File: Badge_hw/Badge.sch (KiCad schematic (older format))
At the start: 133 parts, among them Q1 IRLML9303, Q2 NPN, SW1 SW_PUSH

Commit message: update 9.12 - scheme + case updated
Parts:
- removed ANT1: ANT_PCB_MONO, symbol ANT_PCB_MONO
- removed DD4: STM32L476Rx, LQFP_TQFP:LQFP64, symbol STM32L476Rx
- added D4, D5, D6: LED, symbol LED
- added D7: ANT, symbol ANT
- added DD4: STM32L476Vx, LQFP_TQFP:LQFP100, symbol STM32L476Vx
- added R41: 40kR, symbol R-RESCUE-Badge
- added R42, R43, R44, R45: 1kR, symbol R-RESCUE-Badge
- added R?: Fuse0R, symbol R-RESCUE-Badge
- added SA2, SA3: SW_PUSH, symbol SW_PUSH
- C51, C53: value 18pF -> 18p
- D3: symbol DIODE -> DIODE-RESCUE-Badge
- L1, L2, L3, L4, L5, L6, L7: symbol L -> L-RESCUE-Badge
- R2: value 470R -> 1kR
- R31: value 500R -> 1kR
- R35: value 195 -> 195R
- renumbered SW1 to SA1
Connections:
- net labels added: VGND
- net labels removed: GNDD, GNDPWR, MCU_RST
- wire segments 479 -> 516
- no-connect marks 17 -> 44
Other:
- note added: "Battery"
- note added: "I2C PullUp"
- note added: "LCD"
- note added: "POWOK ?"
- note added: "Power supply"
- note added: "RGB LED"
- note removed: "21"
- note removed: "LED"
- moved on the sheet: C1, C10, C11, C12, C13, C15, C16, C17, C18, C19, C2, C21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

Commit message: 9.2 +pcb
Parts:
- removed D4, D5, D6: LED, symbol LED
- added C67: 10u, Capacitors:CAP_0603, symbol C-RESCUE-Badge
- added D4: LED_RGB, LEDs:LED_5050, symbol LED_RGB-RESCUE-Badge
- added TP1: TESTPOINT, PCB:TESTPOINT_1MM, symbol TESTPOINT
- C1, C10, C11, C12, C13, C14, C15, C16, C17, C18, C19, C2, C20, C21, C22, C23, C24, C25, C26, C27, C28, C29, C3, C30, C31, C32, C33, C34, C35, C36, C37, C38, C39, C4, C40, C41, C42, C43, C44, C45, C46, C47, C48, C49, C50, C51, C52, C53, C54, C55, C56, C57, C58, C59, C6, C60, C61, C62, C63, C65, C66, C7, C8, C9: footprint (none) -> Capacitors:CAP_0603
- C5: value 22u -> 10u; footprint (none) -> Capacitors:CAP_0603
- C64: value 3.9pF -> 3.9pF*; footprint (none) -> Capacitors:CAP_0603
- D1, D2: footprint (none) -> LEDs:LED_0603; symbol LED -> LED-RESCUE-Badge
- D3: footprint (none) -> Diodes:SOD80C
- DA1: footprint (none) -> SO_DIL_TSSOP:SO8_208MIL
- DD1: footprint QFN_DFN:QFN16_4x4_H -> LGA:16_4X4_P065
- DD2: footprint (none) -> Connectors:ER-CON50HT-1
- DD3: footprint (none) -> QFN_DFN:QFN48
- L7: value 12nH -> 12nH*
- LIPO_BAT1: footprint (none) -> Connectors:PLS-2
- Q1: footprint (none) -> SOT:SOT23-3
- Q2: value NPN -> BC848; footprint (none) -> SOT:SOT23-3
- R1, R10, R11, R12, R13, R14, R15, R16, R17, R18, R19, R20, R21, R22, R23, R24, R25, R26, R27, R28, R29, R3, R30, R32, R33, R34, R36, R37, R38, R39, R4, R40, R5, R6, R7, R8, R9: footprint (none) -> Resistors:RES_0603
- R2, R31, R42, R43, R44, R45: value 1kR -> 1k; footprint (none) -> Resistors:RES_0603
- R35: value 195R -> 56k; footprint (none) -> Resistors:RES_0603
- R41: value 40kR -> 51k; footprint (none) -> Resistors:RES_0603
- R46: renamed from R?; footprint (none) -> Resistors:RES_0603_FUSE
- SA1, SA2, SA3: footprint (none) -> BtnsSwitches:BTN_6x6_4x4
- XL1: footprint (none) -> Connectors:PLS-6
- XL2: footprint (none) -> Connectors:USBmicro_MOLEX_WM17142
- XL3: footprint (none) -> Connectors:MICROSD_CAP_FIX05A
- XTAL1: footprint (none) -> Quartz:0503x4-4
- XTAL2: footprint CRYSTAL -> Quartz:0503x4-4
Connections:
- net labels added: +3V3
- wire segments 516 -> 520
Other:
- note removed: "Debug LED"
- note removed: "RGB LED"
- moved on the sheet: BLN1, C1, C10, C11, C12, C13, C15, C17, C18, C19, C2, C21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

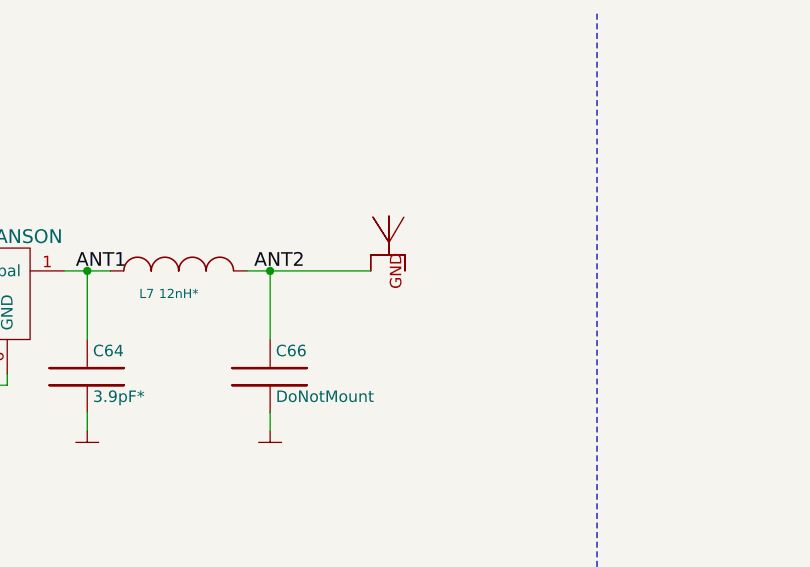
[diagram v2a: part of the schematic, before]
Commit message: +antenna
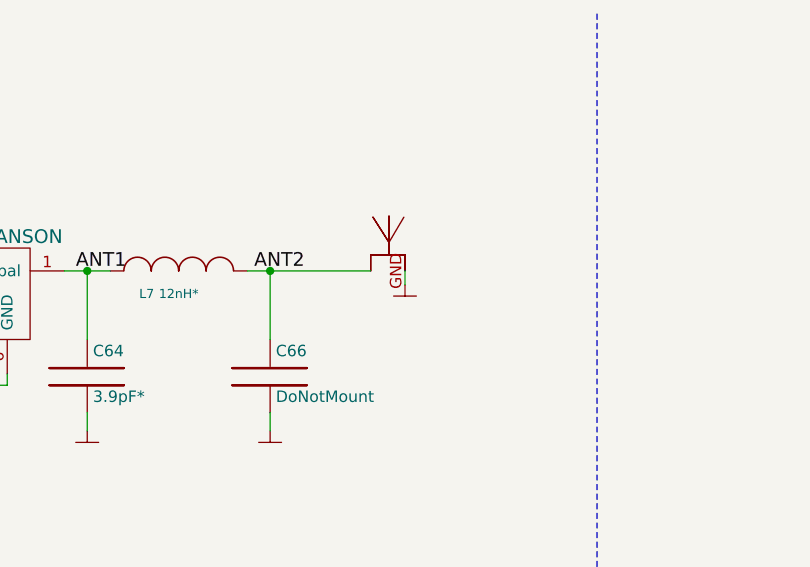
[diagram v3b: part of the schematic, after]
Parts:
- D7: footprint (none) -> ANT_868_INV_F:ANTENNA_868_INV_F
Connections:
- wire segments 520 -> 521
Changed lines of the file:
@@
 LIBS:contrib
 LIBS:valves
-LIBS:ns_power
-LIBS:adc_kl
-LIBS:Allwinner
-LIBS:Antennas_kl
-LIBS:Atmel_kl
-LIBS:Audio_kl
-LIBS:Auds
-LIBS:Connectors_kl
-LIBS:dac
-LIBS:display_kl
-LIBS:ESDProtection
-LIBS:Interface_kl
-LIBS:modules
-LIBS:OpAmp_kl
-LIBS:pcb_details
-LIBS:Power_kl
-LIBS:RF ICs
 LIBS:Sensors
-LIBS:SmartCard_kl
-LIBS:st_kl
-LIBS:standard_logic
 LIBS:Switches
-LIBS:Tittar_kl
-LIBS:Transformers
-LIBS:Transistors_kl
 LIBS:Badge-cache1
 LIBS:Badge-cacheGOST
-LIBS:ns_antennas
 LIBS:Badge-cache
 EELAYER 26 0
@@
 F 0 "D7" H 24570 1785 60  0001 C CNN
 F 1 "ANT" H 24365 1815 60  0001 C CNN
-F 2 "" H 24470 1530 60  0001 C CNN
+F 2 "ANT_868_INV_F:ANTENNA_868_INV_F" H 24470 1530 60  0001 C CNN
 F 3 "" H 24470 1530 60  0001 C CNN
 	1    24470 1530
@@
 	1    0    0    -1
 $EndComp
+$Comp
+L GNDSignal #PWR?
+U 1 1 589CC065
+P 24620 1660
+F 0 "#PWR?" H 24670 1710 50  0001 C CNN
+F 1 "GNDSignal" H 20  -190 50  0001 C CNN
+F 2 "" H 20  -90 50  0000 C CNN
+F 3 "" H 20  -90 50  0000 C CNN
+	1    24620 1660
+	1    0    0    -1
+$EndComp
+Wire Wire Line
+	24620 1660 24620 1600
 $EndSCHEMATC

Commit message: * pcb redraw + barometer scheme
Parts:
- added C68: 0.1u, Capacitors:CAP_0603, symbol C-RESCUE-Badge
- added DD6: LPS22HB, QFN_DFN:QFN16_4x4_H, symbol LPS22HB
- added L8: BLM15AG102, Inductors:IND_0402, symbol L-RESCUE-Badge
- C64, C66: footprint Capacitors:CAP_0603 -> Capacitors:CAP_0402
- D7: footprint ANT_868_INV_F:ANTENNA_868_INV_F -> ANT_868_INV_F:ANTENNA_868_INV_F_SHARP
- DD1: footprint LGA:16_4X4_P065 -> QFN_DFN:QFN16_4x4_H
- L1, L3, L4: footprint Inductors:IND_0402 -> Inductors:SDR0805
- L6: footprint Inductors:IND_0402 -> Inductors:IND_SDR0604
- LIPO_BAT1: footprint Connectors:PLS-2 -> Connectors:WB-02(MW-2M)
- R15: footprint Resistors:RES_0603 -> Resistors:RES_1206
- XTAL2: footprint Quartz:0503x4-4 -> Quartz:03225C4
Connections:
- net labels added: PRESSURE_INT
- net labels removed: DCDC_3
- wire segments 521 -> 539
- no-connect marks 44 -> 43
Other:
- note added: "0R03 footprint?"
- note added: "?? Resistor\non I2C_en"
- note added: "???"
- note added: "Barometer"
- moved on the sheet: C44, C46, C49, C50, C52, C55, C58, C63, C65, D3, DA1A, DA1B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
